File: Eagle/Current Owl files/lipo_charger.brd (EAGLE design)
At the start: 68.6 x 47 mm, 23 parts, among them J1 2X6 FEMALE, J2 2X6 FEMALE, Q1 2N3906, X1 SMA-142-0701-851/861

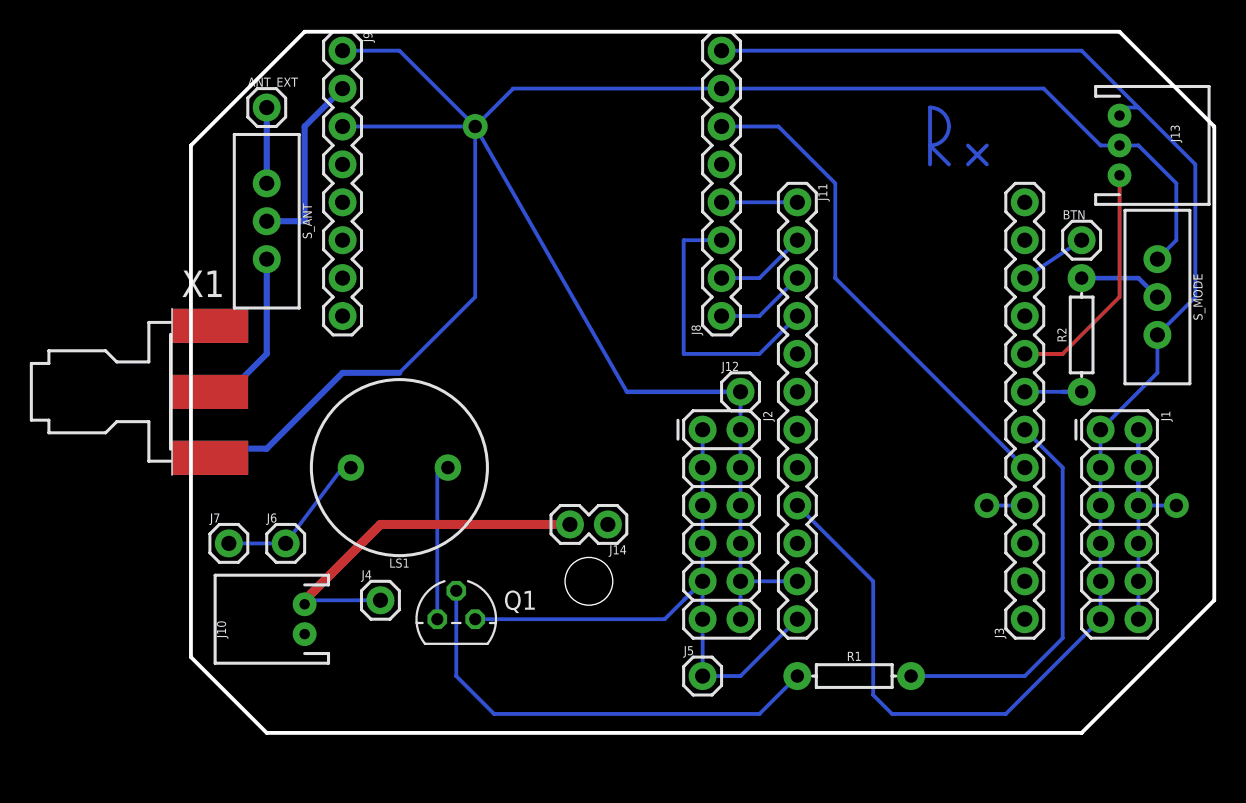
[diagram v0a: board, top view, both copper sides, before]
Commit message: updated eagle files
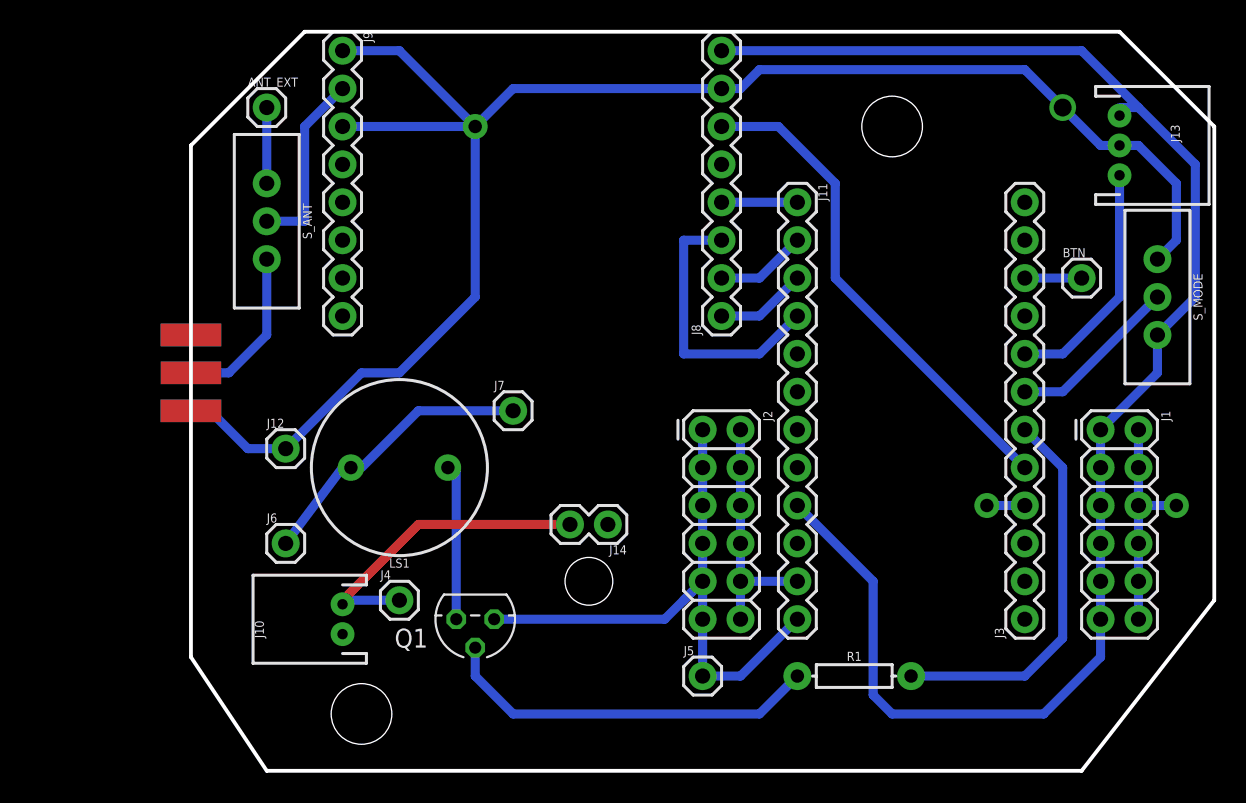
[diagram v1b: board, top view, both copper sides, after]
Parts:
- removed R2: 10k, SparkFun-Resistors:AXIAL-0.3
- removed X1: SMA-142-0701-851/861, con-coax:J502-ND-142-0701-851/861
- added J$1: SMA_EDGE, SparkFun-Retired:SMA-EDGE
- moved J12 30.7 mm to (6.35, 17.8)
- moved J7 21.0 mm to (21.6, 20.3)
- moved J10 2.54 mm to (10.2, 6.35)
- moved BTN 2.54 mm to (59.7, 29.2)
- moved J4 1.27 mm to (14.0, 7.62)
- moved Q1 1.27 mm to (19.1, 6.35), turned to 180 degrees
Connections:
- removed net 7: J3.7, R2.P$1
- net GND: now also J$1.GND@0, J$1.GND@1, J$1.GND@2, J$1.GND@3; no longer X1.G@1, X1.G@2, X1.G@3, X1.G@4
- net N$3: now also Q1.1; no longer Q1.3
- net N$6: now also J3.7; no longer R2.P$2
- net N$8: now also J$1.SIG; no longer X1.1
- net RAW: now also Q1.3; no longer Q1.1
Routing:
- net GND: track 178.3 -> 151.1 mm, vias 3 -> 4
- net N$2: track 9.20 -> 0.00 mm
- net N$11: track 10.2 -> 18.1 mm
- net N$6: track 5.61 -> 11.5 mm
- net N$1: track 30.0 -> 25.0 mm
- net 7: track 3.81 -> 0.00 mm
- net N$9: track 19.9 -> 17.3 mm
- net N$5: track 1.80 -> 0.00 mm
- net N$4: track 1.80 -> 0.00 mm
- net VCC: track 102.5 -> 104.0 mm
- net N$10: track 5.08 -> 3.81 mm
- net RAW: track 42.5 -> 41.3 mm
- net 10: track 4.58 -> 3.81 mm
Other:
- board size 68.6 x 47 mm -> 68.6 x 49.5 mm
